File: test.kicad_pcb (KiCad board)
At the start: 2 copper layers, 110 x 100 mm, 218 parts, among them J1 HSP2_MX-502584-0670, J10 Gniazdo programatora SWD, J11 Gniazdo akumulatora, J12 Gniazdo akumulatora, J13 SIMHOLDER, J14 BTN1, J15 BTN2, J2 HSP2_MX-502584-0670, J3 HSP2_MX-502584-0670, J4 HSP2_MX-502584-0670, J5 HSP2_MX-502584-0670, J6 HSP2_MX-502584-0670, J7 CONN_02X01, J8 CONN_02X01, J9 microSD, T1 IRLML6401, T10 BSS138, T11 BSS138, T12 BSS138, T13 BSS138, T14 FDV304P, T2 IRLML6401, T3 IRLML6401, T4 IRLML6401, T5 IRLML6401, T6 IRLML6401, T7 BSS138, T8 BSS138, T9 BSS138, U1 MCP1755T-3302E/DC, U10 TPS3823, U11 STM32L051R8, U12 DS3231SN, U13 MCP1755T-3302E/DC, U14 MCP1755T-3302E/DC, U15 MIC29302, U16 DHT22, U17 M590E, U18 AT45DB161E-SSHD-T, U19 ESP-WROOM-32, U2 MCP1755T-3302E/DC, U3 MCP1755T-3302E/DC, U4 MCP1755T-3302E/DC, U5 MCP1755T-3302E/DC, U6 MCP1755T-3302E/DC, U7 74LVX373M, U8 74LVX373M, U9 MAX3485, Y1 32.768 kHz, Y2 8 MHz

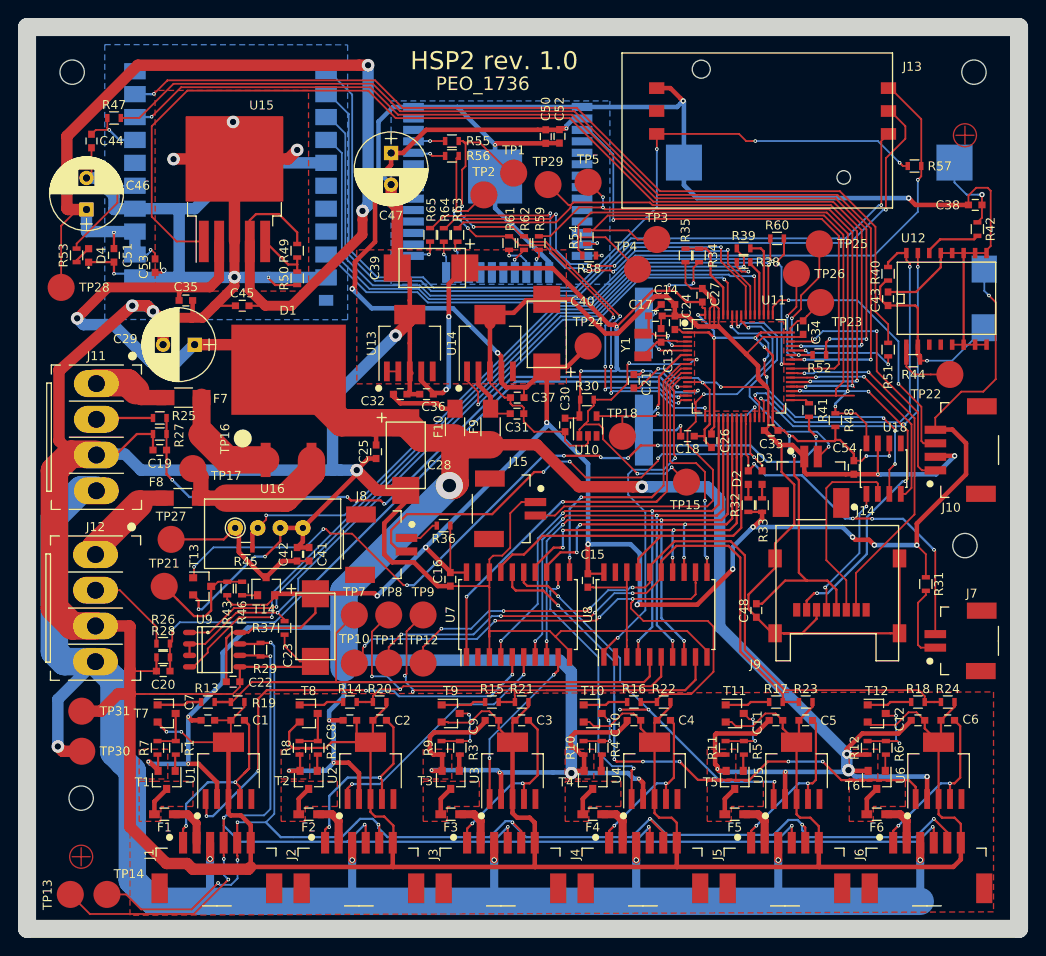
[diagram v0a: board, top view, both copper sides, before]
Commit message: poprawione przelotki i ścieżki
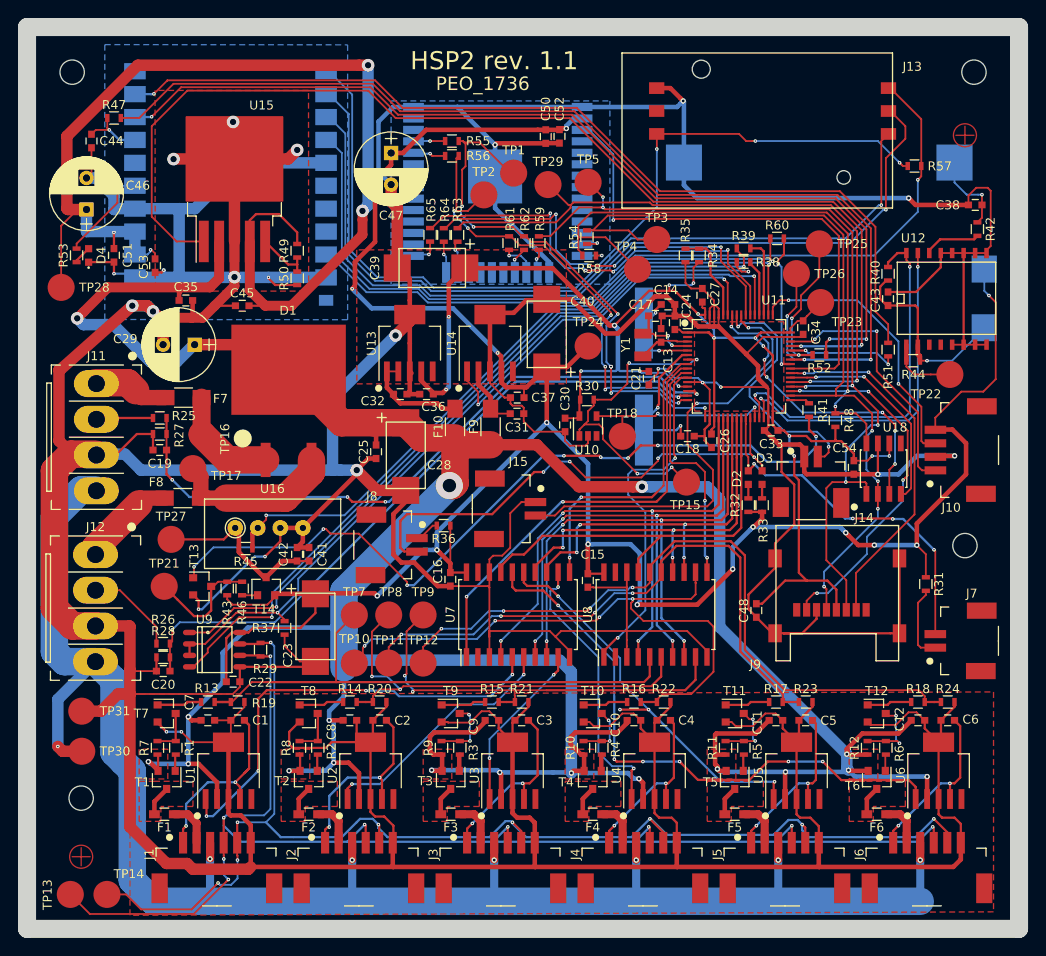
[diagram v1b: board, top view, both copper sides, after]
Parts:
- moved C21 1.70 mm to (167.9, 88.9)
- moved J8 1.16 mm to (135.5, 103.2)
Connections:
- U18 pad 1: /SPI_CLK -> /SPI_MOSI
- U18 pad 2: /SPI_MOSI -> /SPI_CLK
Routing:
- net /SPI_CLK: track 77.6 -> 90.7 mm, vias 2 -> 4
- net /SPI_MOSI: track 86.6 -> 98.8 mm, vias 4 -> 6
- net Net-(C32-Pad1): track 9.83 -> 12.7 mm
- net GND: track 1114.5 -> 1112.0 mm
- net +3.3V: track 274.6 -> 273.1 mm
- net Net-(D3-Pad1): track 56.1 -> 55.0 mm
- net Net-(C14-Pad1): track 11.6 -> 12.2 mm
- net /I2C2_SDA: track 39.2 -> 38.6 mm
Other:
- board text added: "HSP2 rev. 1.1"
- board text removed: "HSP2 rev. 1.0"
